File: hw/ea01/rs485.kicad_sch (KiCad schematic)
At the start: 1 part, among them U12 SN75176AP

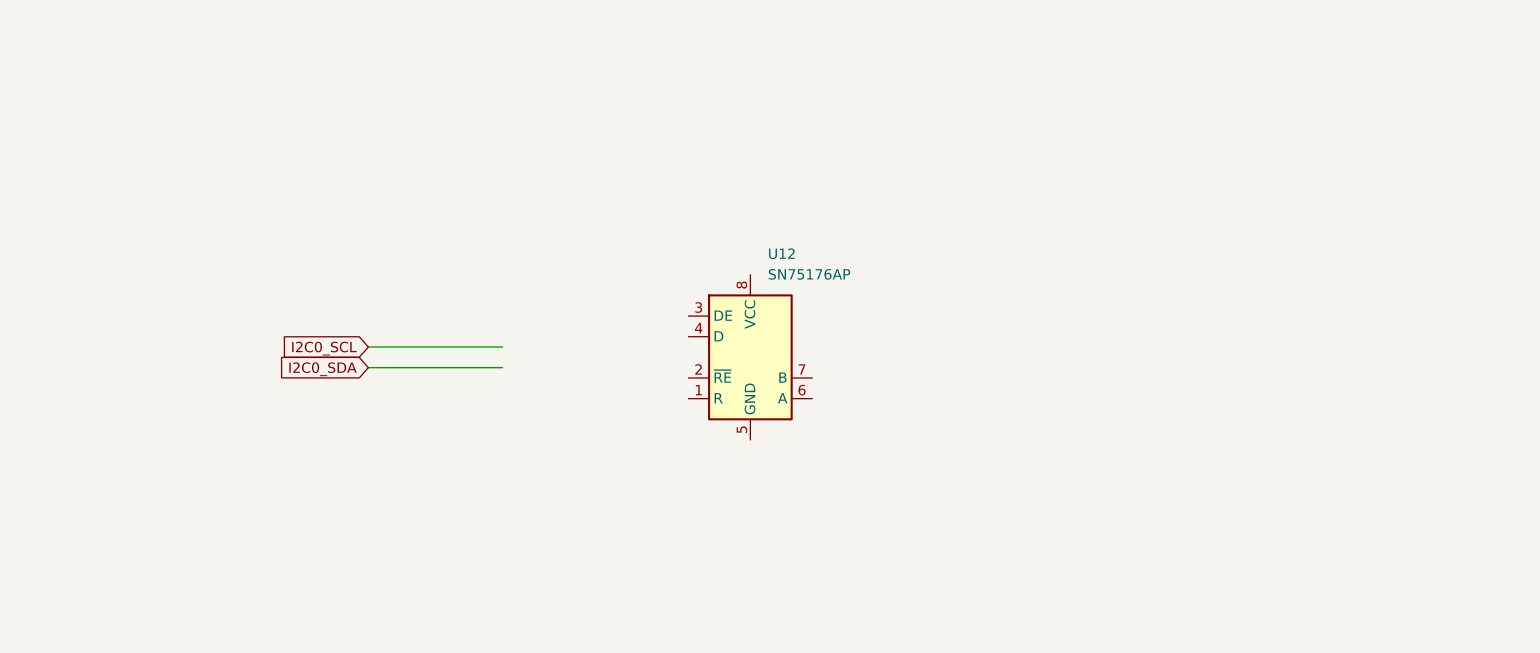
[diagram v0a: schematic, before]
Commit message: schmatic drawing continue...
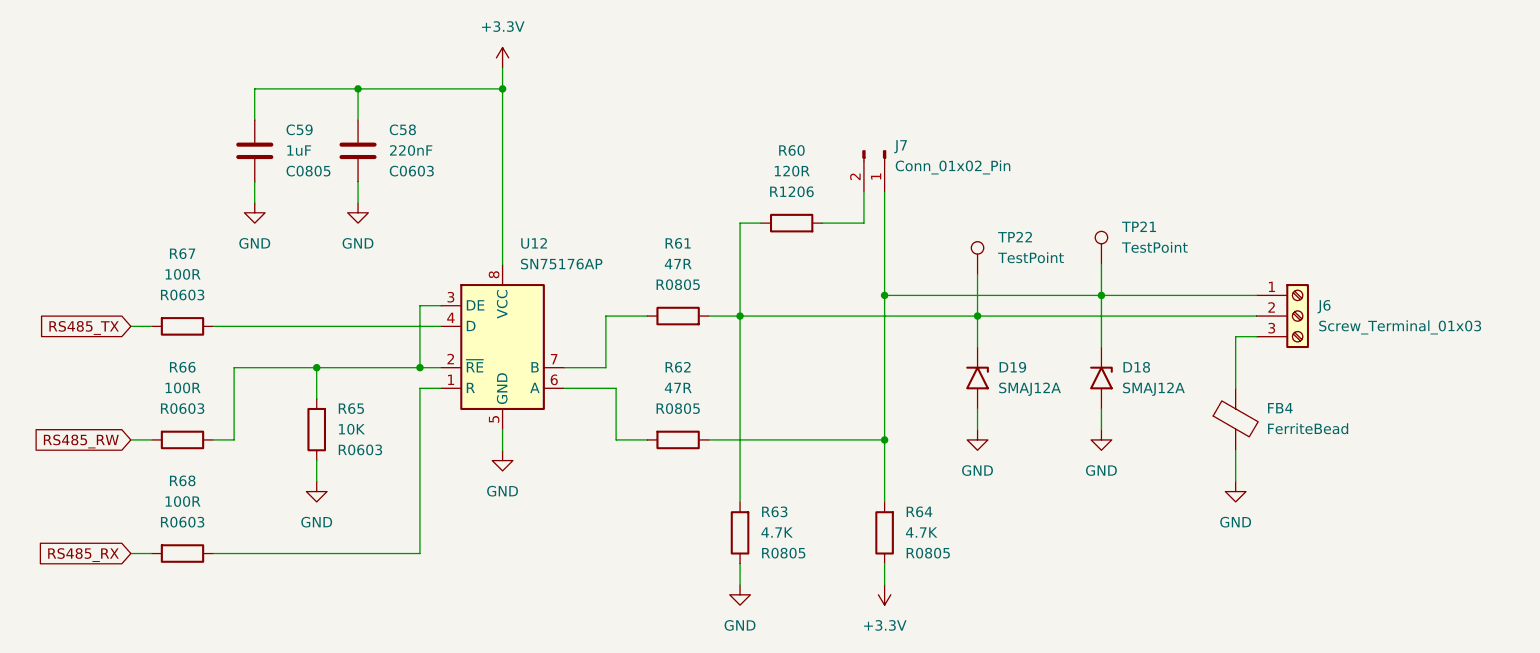
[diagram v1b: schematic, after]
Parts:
- added C58: 220nF, Capacitor_SMD:C_0603_1608Metric, symbol Device:C
- added C59: 1uF, Capacitor_SMD:C_0805_2012Metric, symbol Device:C
- added D18, D19: SMAJ12A, Diode_SMD:D_SMA, symbol Diode:SMAJ24A
- added FB4: FerriteBead, symbol Device:FerriteBead
- added J6: Screw_Terminal_01x03, symbol Connector:Screw_Terminal_01x03
- added J7: Conn_01x02_Pin, symbol Connector:Conn_01x02_Pin
- added R60: 120R, Resistor_SMD:R_1206_3216Metric, symbol Device:R
- added R61, R62: 47R, Resistor_SMD:R_0805_2012Metric, symbol Device:R
- added R63, R64: 4.7K, Resistor_SMD:R_0805_2012Metric, symbol Device:R
- added R65: 10K, Resistor_SMD:R_0603_1608Metric, symbol Device:R
- added R66, R67, R68: 100R, Resistor_SMD:R_0603_1608Metric, symbol Device:R
- added TP21, TP22: TestPoint, TestPoint:TestPoint_Pad_D1.5mm, symbol Connector:TestPoint
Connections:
- net at U12.1 (R): now also R68.1
- net at U12.2 (~{RE}): now also U12.3 (DE), R65.2, R66.1
- net at U12.4 (D): now also R67.1
- net GND: now reaches U12.5 (GND)
- net GND: now also C58.2, C59.2, D18.2 (A2), D19.2 (A2), FB4.2, R63.1, R65.1
- net at U12.6 (A): now also R62.2
- net at U12.7 (B): now also R61.1
- net +3.3V: now reaches U12.8 (VCC)
- net +3.3V: now also C58.1, C59.1, R64.1
- new net: D18.1 (A1), J6.1 (Pin_1), J7.1 (Pin_1), R62.1, R64.2, TP21.1
- new net: J7.2 (Pin_2), R60.2
- new net: D19.1 (A1), J6.2 (Pin_2), R60.1, R61.2, R63.2, TP22.1
- new net: FB4.1, J6.3 (Pin_3)
- new net RS485_RW: R66.2
- new net RS485_RX: R68.2
- new net RS485_TX: R67.2
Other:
- moved on the sheet: U12
